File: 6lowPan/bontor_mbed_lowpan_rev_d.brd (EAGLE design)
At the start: 98 x 107 mm, 170 parts, among them IC1 SIM900, IC2 74HC595D, IC3 74HC595D, IC4 ADE7758RW, IC5 74HC595D, J1 U.FL, U2 W5500, X1 NX2520SA

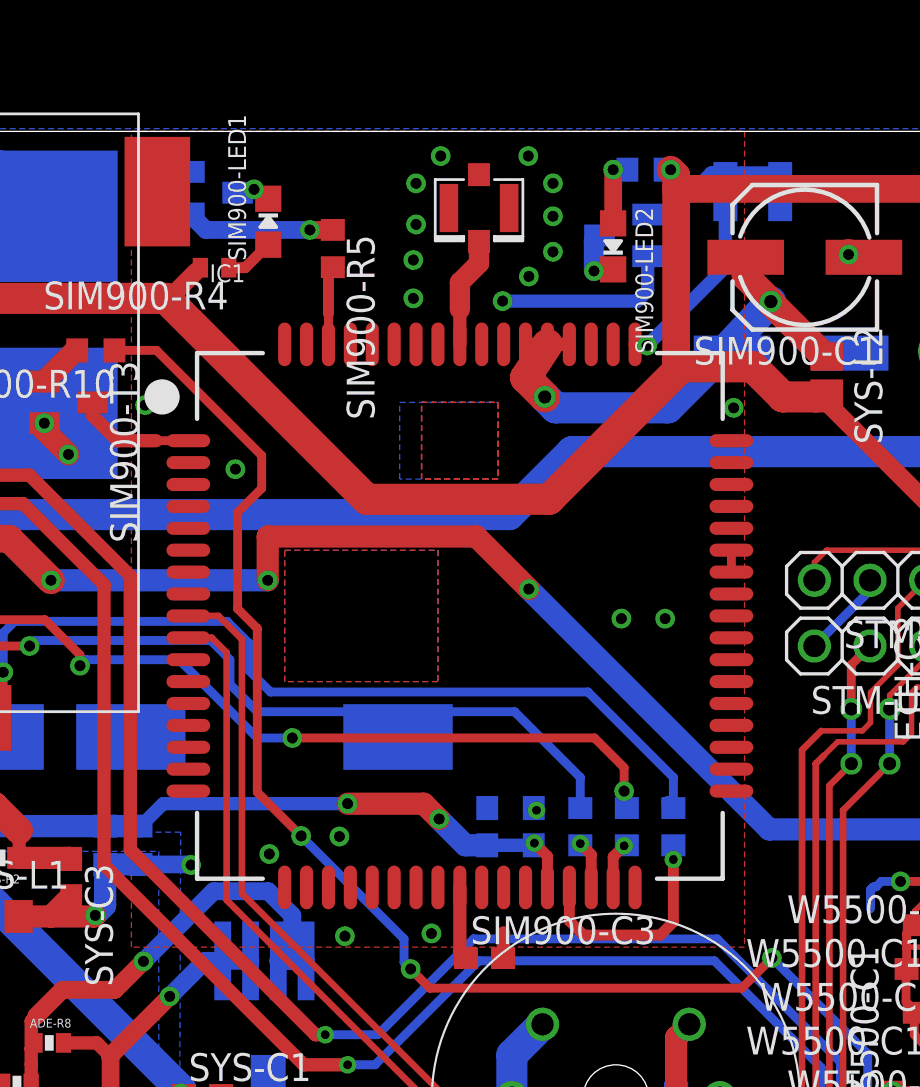
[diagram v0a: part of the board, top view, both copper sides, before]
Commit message: add gerber and BoM
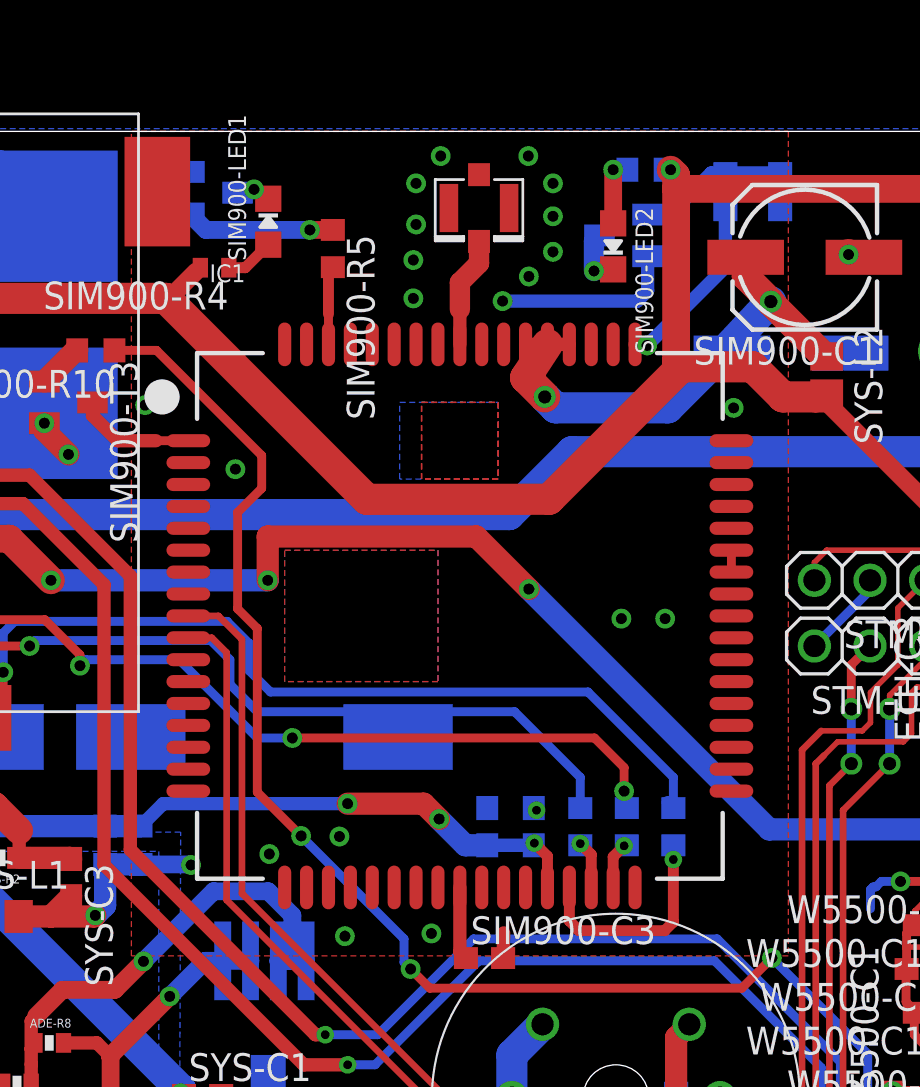
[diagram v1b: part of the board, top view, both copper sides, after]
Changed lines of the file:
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@@
 <setting verticaltext="up"/>
 </settings>
-<grid distance="0.1" unitdist="mm" unit="mm" style="lines" multiple="1" display="yes" altdistance="0.125" altunitdist="mm" altunit="mm"/>
+<grid distance="1" unitdist="mm" unit="mm" style="lines" multiple="1" display="yes" altdistance="0.125" altunitdist="mm" altunit="mm"/>
 <layers>
 <layer number="1" name="Top" color="4" fill="1" visible="yes" active="yes"/>
@@
 <polygon width="0.254" layer="1" isolate="0.4064">
 <vertex x="40.25" y="107"/>
-<vertex x="68.25" y="107"/>
-<vertex x="68.25" y="69.75"/>
-<vertex x="40.25" y="69.75"/>
+<vertex x="70.25" y="107"/>
+<vertex x="70.25" y="69.35"/>
+<vertex x="40.25" y="69.35"/>
 </polygon>
 <via x="58.75" y="76" extent="1-16" drill="0.4"/>
@@
 <via x="36.275" y="93.675" extent="1-16" drill="0.5"/>
 <wire x1="36.275" y1="93.675" x2="36.275" y2="93.35" width="1.016" layer="1"/>
-<wire x1="57.25" y1="70.4" x2="53.95" y2="70.375" width="0" layer="19" extent="1-1"/>
 </signal>
 <signal name="VDD">
@@
 <wire x1="65" y1="73.75" x2="65" y2="74.4" width="0.4064" layer="16"/>
 <wire x1="60.25" y1="72.475" x2="60.25" y2="70.95" width="0.5" layer="1"/>
-<wire x1="60.25" y1="70.95" x2="60.9" y2="70.3" width="0.5" layer="1"/>
-<wire x1="60.9" y1="70.3" x2="64.4" y2="70.3" width="0.5" layer="1"/>
-<wire x1="64.4" y1="70.3" x2="65" y2="70.9" width="0.5" layer="1"/>
 <wire x1="65" y1="70.9" x2="65" y2="73.75" width="0.5" layer="1"/>
+<wire x1="60.25" y1="70.95" x2="60.7" y2="70.5" width="0.5" layer="1"/>
+<wire x1="60.7" y1="70.5" x2="64.6" y2="70.5" width="0.5" layer="1"/>
+<wire x1="64.6" y1="70.5" x2="65" y2="70.9" width="0.5" layer="1"/>
 </signal>
 <signal name="N$8">
